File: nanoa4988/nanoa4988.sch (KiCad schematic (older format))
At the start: 12 parts, among them J1 Conn_01x04, J2 Conn_01x04, J3 Conn_01x04, J4 Conn_01x02

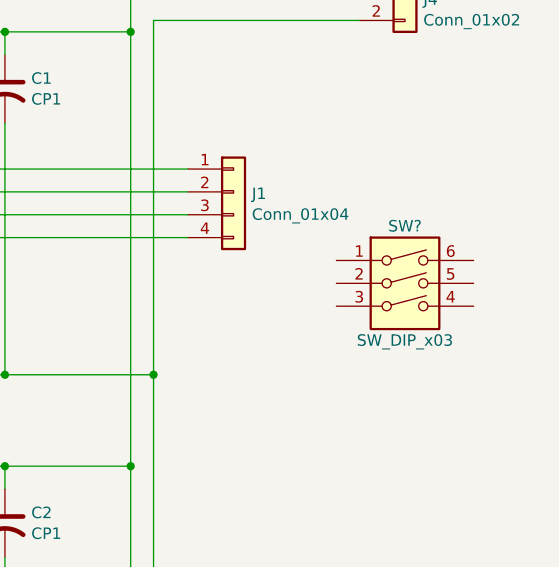
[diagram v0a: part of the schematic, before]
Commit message: Further Cleanup
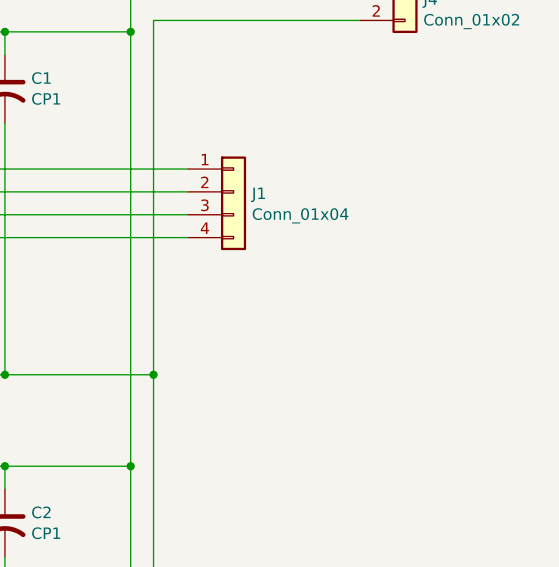
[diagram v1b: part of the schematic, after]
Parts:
- removed SW?: SW_DIP_x03, symbol nanoa4988-rescue:SW_DIP_x03-RESCUE-nanoa4988
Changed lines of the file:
@@
 Wire Wire Line
 	3400 3300 3800 3300
-$Comp
-L nanoa4988-rescue:SW_DIP_x03-RESCUE-nanoa4988 SW?
-U 1 1 5ABE8311
-P 8050 2200
-F 0 "SW?" H 8050 2550 50  0000 C CNN
-F 1 "SW_DIP_x03" H 8050 2050 50  0000 C CNN
-F 2 "" H 8050 2200 50  0001 C CNN
-F 3 "" H 8050 2200 50  0001 C CNN
-	1    8050 2200
-	1    0    0    -1
-$EndComp
 $EndSCHEMATC

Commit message: Cleaned directories
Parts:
- A1: symbol nanoa4988-rescue:MCU_Module_Arduino_Nano_v3.x-RESCUE-nanoa4988 -> MCU_Module:Arduino_Nano_v3.x
- A2, A3, A4: symbol nanoa4988-rescue:Driver_Motor_Pololu_Breakout_A4988-RESCUE-nanoa4988 -> Driver_Motor:Pololu_Breakout_A4988
- C1, C2, C3: symbol nanoa4988-rescue:Device_CP1-RESCUE-nanoa4988 -> Device:CP1
- J1, J2, J3: symbol nanoa4988-rescue:Connector_Generic_Conn_01x04-RESCUE-nanoa4988 -> Connector_Generic:Conn_01x04
- J4: symbol nanoa4988-rescue:Connector_Generic_Conn_01x02-RESCUE-nanoa4988 -> Connector_Generic:Conn_01x02
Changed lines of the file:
@@
 EESchema Schematic File Version 4
-LIBS:nanoa4988-cache
 EELAYER 26 0
 EELAYER END
@@
 $EndDescr
 $Comp
-L nanoa4988-rescue:MCU_Module_Arduino_Nano_v3.x-RESCUE-nanoa4988 A1
+L MCU_Module:Arduino_Nano_v3.x A1
 U 1 1 5AB0D5C3
 P 2900 3200
@@
 $EndComp
 $Comp
-L nanoa4988-rescue:Driver_Motor_Pololu_Breakout_A4988-RESCUE-nanoa4988 A2
+L Driver_Motor:Pololu_Breakout_A4988 A2
 U 1 1 5AB0D6AA
 P 5650 1700
@@
 $EndComp
 $Comp
-L nanoa4988-rescue:Driver_Motor_Pololu_Breakout_A4988-RESCUE-nanoa4988 A3
+L Driver_Motor:Pololu_Breakout_A4988 A3
 U 1 1 5AB0D71C
 P 5650 3600
@@
 $EndComp
 $Comp
-L nanoa4988-rescue:Driver_Motor_Pololu_Breakout_A4988-RESCUE-nanoa4988 A4
+L Driver_Motor:Pololu_Breakout_A4988 A4
 U 1 1 5AB0D791
 P 5650 5700
@@
 $EndComp
 $Comp
-L nanoa4988-rescue:Device_CP1-RESCUE-nanoa4988 C1
+L Device:CP1 C1
 U 1 1 5AB0D835
 P 6300 1250
@@
 $EndComp
 $Comp
-L nanoa4988-rescue:Device_CP1-RESCUE-nanoa4988 C2
+L Device:CP1 C2
 U 1 1 5AB0D932
 P 6300 3150
@@
 $EndComp
 $Comp
-L nanoa4988-rescue:Device_CP1-RESCUE-nanoa4988 C3
+L Device:CP1 C3
 U 1 1 5AB0D9D4
 P 6300 5250
@@
 $EndComp
 $Comp
-L nanoa4988-rescue:Connector_Generic_Conn_01x04-RESCUE-nanoa4988 J1
+L Connector_Generic:Conn_01x04 J1
 U 1 1 5AB0DB82
 P 7300 1700
@@
 $EndComp
 $Comp
-L nanoa4988-rescue:Connector_Generic_Conn_01x04-RESCUE-nanoa4988 J2
+L Connector_Generic:Conn_01x04 J2
 U 1 1 5AB0DC34
 P 7300 3600
@@
 $EndComp
 $Comp
-L nanoa4988-rescue:Connector_Generic_Conn_01x04-RESCUE-nanoa4988 J3
+L Connector_Generic:Conn_01x04 J3
 U 1 1 5AB0DC9B
 P 7300 5700
@@
 $EndComp
 $Comp
-L nanoa4988-rescue:Connector_Generic_Conn_01x02-RESCUE-nanoa4988 J4
+L Connector_Generic:Conn_01x02 J4
 U 1 1 5AB0DE10
 P 8050 850
